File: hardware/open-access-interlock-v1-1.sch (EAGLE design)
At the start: 19 parts

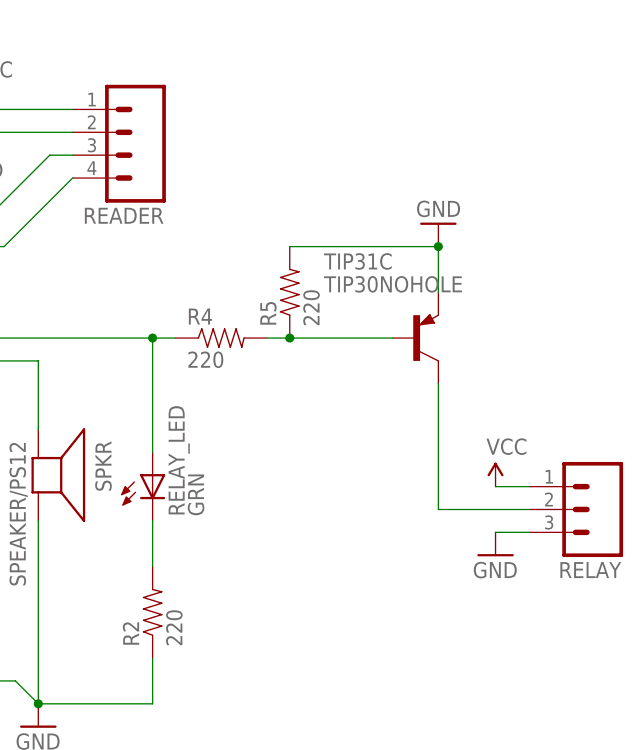
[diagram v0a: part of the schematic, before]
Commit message: Fixing transistor/relay stuff
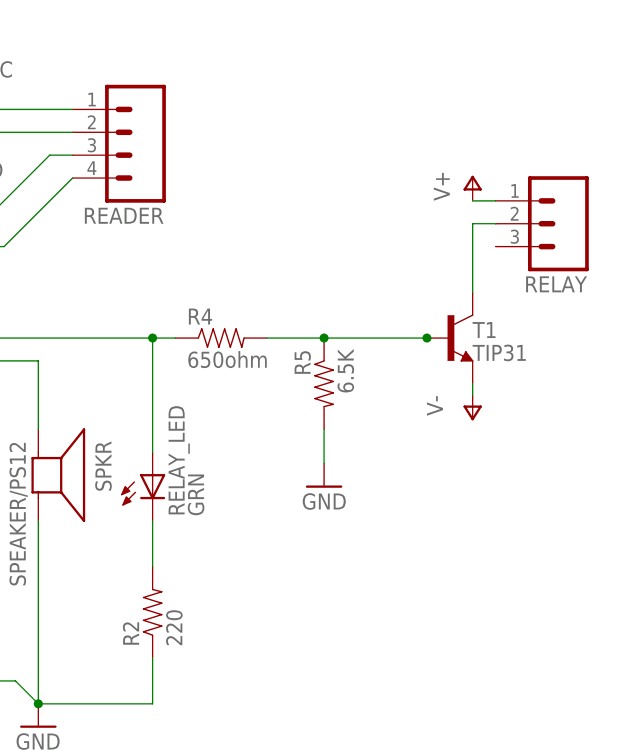
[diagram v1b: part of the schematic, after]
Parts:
- removed TIP31C: TIP30NOHOLE, adafruit:TIP30NOHOLE
- added T1: TIP31, transistor:TIP31
- R4: value 220 -> 650ohm
- R5: value 220 -> 6.5K
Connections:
- new net V+: RELAY.1
- new net V-: T1.E
- net GND: no longer RELAY.3, TIP31C.E
- net N$13: now also T1.C; no longer TIP31C.C
- net N$21: now also T1.B; no longer TIP31C.B
- net VCC: no longer RELAY.1
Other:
- moved on the sheet: R5, RELAY
